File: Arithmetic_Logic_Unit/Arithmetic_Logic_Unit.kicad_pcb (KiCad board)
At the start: 2 copper layers, 95.9 x 90.2 mm, 81 parts, among them J1 PC104, U1 74LS245, U10 74LS245, U11 74LS173, U15 74LS245, U16 74LS173, U17 74LS173, U2 74LS173, U3 74LS173, U4 74LS08, U5 74LS86, U6 74LS86, U7 74LS02, U8 74LS283, U9 74LS283

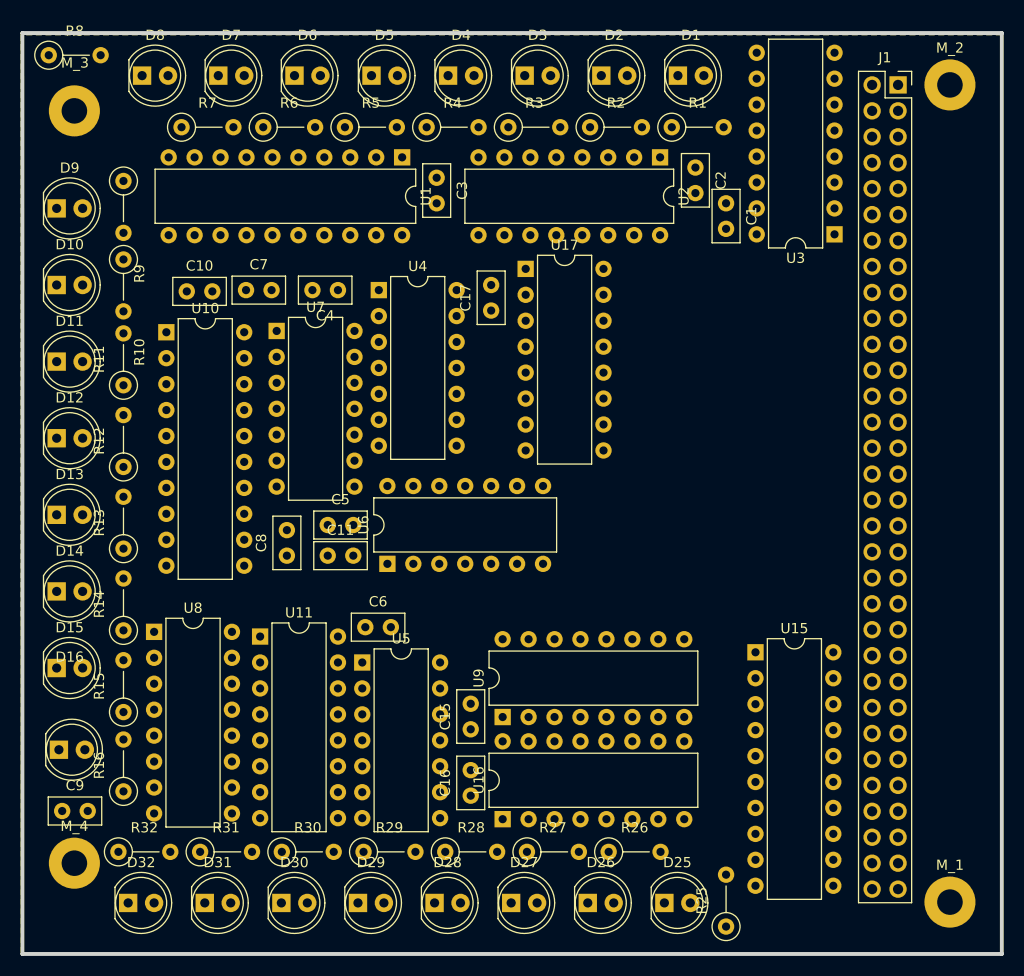
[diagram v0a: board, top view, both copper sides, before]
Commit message: layed out PCB
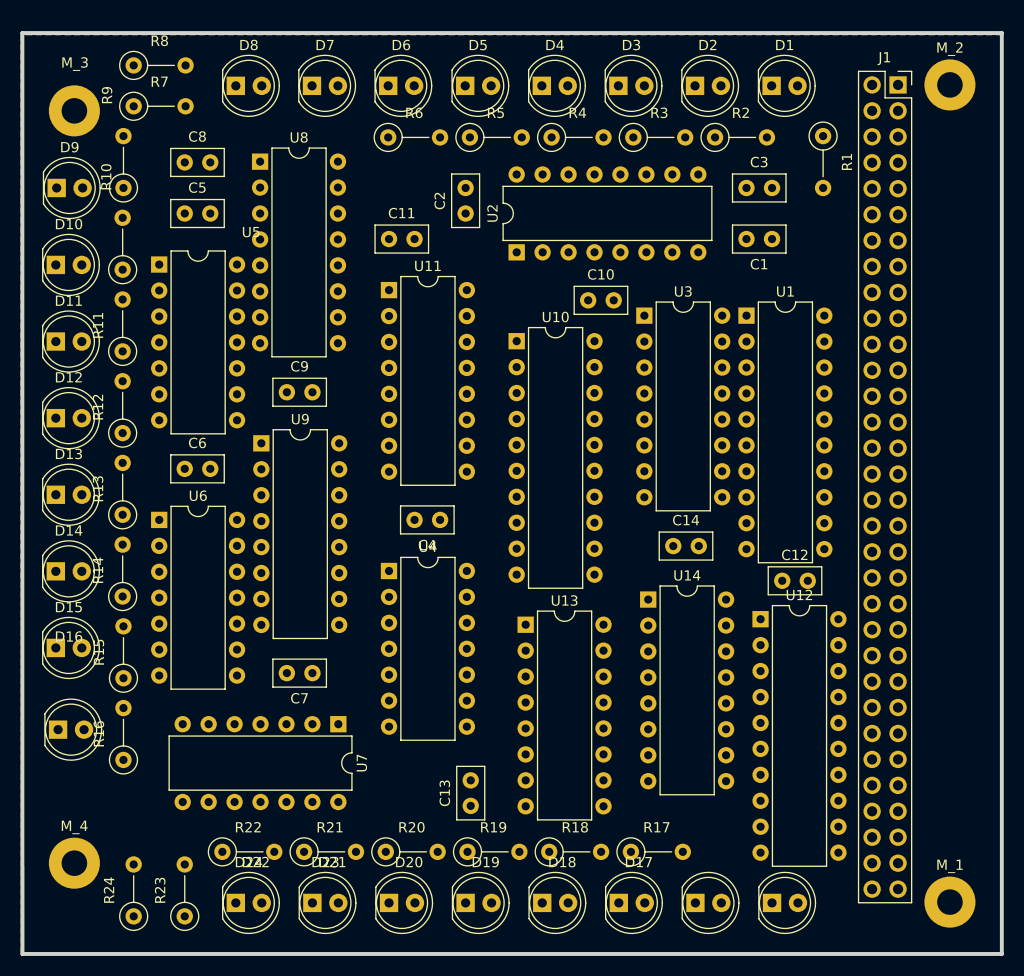
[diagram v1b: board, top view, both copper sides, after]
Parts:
- removed C15, C16, C17: .01µF, Capacitor_THT:C_Disc_D5.0mm_W2.5mm_P2.50mm
- removed D25, D26, D27, D28, D29, D30, D31, D32: LED, LED_THT:LED_D5.0mm
- removed R25, R26, R27, R28, R29, R30, R31, R32: 220, Resistor_THT:R_Axial_DIN0207_L6.3mm_D2.5mm_P5.08mm_Vertical
- removed U15: 74LS245, Package_DIP:DIP-20_W7.62mm
- removed U16, U17: 74LS173, Package_DIP:DIP-16_W7.62mm
- added C12: .01µF, Capacitor_THT:C_Disc_D5.0mm_W2.5mm_P2.50mm, F.Cu at (156.3, 90.5)
- added C13: .01µF, Capacitor_THT:C_Disc_D5.0mm_W2.5mm_P2.50mm, F.Cu at (125.8, 112.5)
- added C14: .01µF, Capacitor_THT:C_Disc_D5.0mm_W2.5mm_P2.50mm, F.Cu at (145.6, 87.1)
- added D17: LED, LED_THT:LED_D5.0mm, F.Cu at (155.3, 122.0)
- added D18: LED, LED_THT:LED_D5.0mm, F.Cu at (147.8, 122.0)
- added D19: LED, LED_THT:LED_D5.0mm, F.Cu at (140.3, 122.0)
- added D20: LED, LED_THT:LED_D5.0mm, F.Cu at (132.8, 122.0)
- added D21: LED, LED_THT:LED_D5.0mm, F.Cu at (125.3, 122.0)
- added D22: LED, LED_THT:LED_D5.0mm, F.Cu at (117.8, 122.0)
- added D23: LED, LED_THT:LED_D5.0mm, F.Cu at (110.3, 122.0)
- added D24: LED, LED_THT:LED_D5.0mm, F.Cu at (102.8, 122.0)
- added R17: 220, Resistor_THT:R_Axial_DIN0207_L6.3mm_D2.5mm_P5.08mm_Vertical, F.Cu at (141.5, 117.0)
- added R18: 220, Resistor_THT:R_Axial_DIN0207_L6.3mm_D2.5mm_P5.08mm_Vertical, F.Cu at (133.5, 117.0)
- added R19: 220, Resistor_THT:R_Axial_DIN0207_L6.3mm_D2.5mm_P5.08mm_Vertical, F.Cu at (125.5, 117.0)
- added R20: 220, Resistor_THT:R_Axial_DIN0207_L6.3mm_D2.5mm_P5.08mm_Vertical, F.Cu at (117.5, 117.0)
- added R21: 220, Resistor_THT:R_Axial_DIN0207_L6.3mm_D2.5mm_P5.08mm_Vertical, F.Cu at (109.5, 117.0)
- added R22: 220, Resistor_THT:R_Axial_DIN0207_L6.3mm_D2.5mm_P5.08mm_Vertical, F.Cu at (101.5, 117.0)
- added R23: 220, Resistor_THT:R_Axial_DIN0207_L6.3mm_D2.5mm_P5.08mm_Vertical, F.Cu at (97.8, 123.3)
- added R24: 220, Resistor_THT:R_Axial_DIN0207_L6.3mm_D2.5mm_P5.08mm_Vertical, F.Cu at (92.8, 123.3)
- added U12: 74LS245, Package_DIP:DIP-20_W7.62mm, F.Cu at (154.2, 94.2)
- added U13: 74LS173, Package_DIP:DIP-16_W7.62mm, F.Cu at (131.2, 94.8)
- added U14: 74LS173, Package_DIP:DIP-16_W7.62mm, F.Cu at (143.2, 92.3)
- moved U8 47.2 mm to (105.2, 49.4)
- moved C9 46.5 mm to (107.8, 72.0)
- moved U5 43.7 mm to (95.3, 59.5)
- moved C8 39.8 mm to (97.8, 49.5), turned to 0 degrees
- moved C10 39.3 mm to (137.3, 63.0)
- moved U7 39.0 mm to (112.8, 104.5), turned to -90 degrees
- moved C7 38.1 mm to (110.3, 99.5), turned to 180 degrees
- moved U1 37.1 mm to (152.8, 64.5), turned to 0 degrees
- moved U11 36.2 mm to (117.8, 62.0)
- moved U9 35.7 mm to (105.3, 77.0), turned to 0 degrees
- moved U10 34.3 mm to (130.3, 67.0)
- moved C5 33.6 mm to (97.8, 54.5)
- moved C11 31.6 mm to (117.8, 57.0)
- moved C3 30.4 mm to (152.8, 52.0), turned to 0 degrees
- moved U4 27.5 mm to (117.8, 89.5)
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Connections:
- D10 pad 2: /ALU/s6 -> /ALU/s1
- D11 pad 2: /ALU/s5 -> /ALU/s2
- D12 pad 2: /ALU/s4 -> /ALU/s3
- D13 pad 2: /ALU/s3 -> /ALU/s4
- D14 pad 2: /ALU/s2 -> /ALU/s5
- D15 pad 2: /ALU/s1 -> /ALU/s6
- D16 pad 2: /ALU/s0 -> /ALU/s7
- D9 pad 2: /ALU/s7 -> /ALU/s0
